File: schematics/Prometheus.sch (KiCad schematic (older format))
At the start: 15 parts, among them J1 ATX Power Conn, SW2 Power Switch, U1 wdc65c816, U2 DS1501YN, X1 8MHz, X2 32kHz

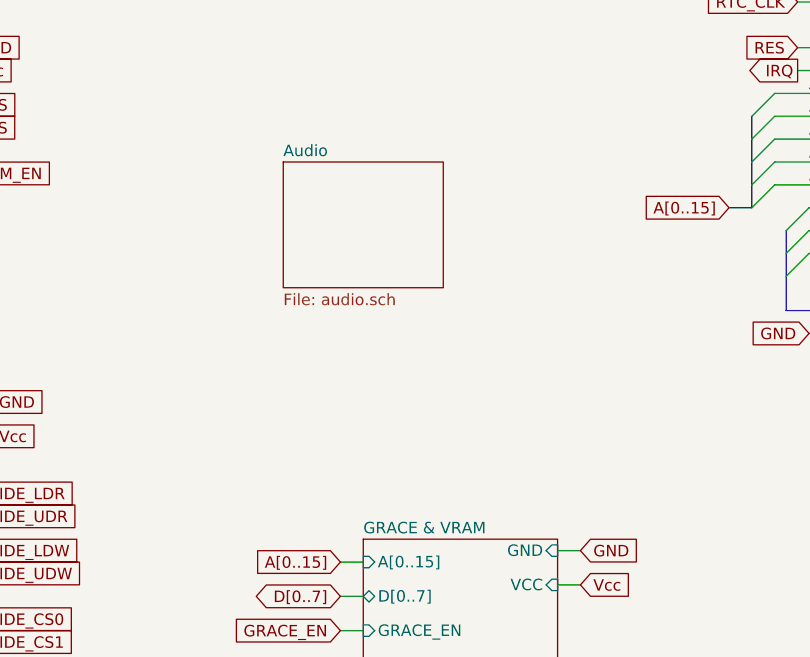
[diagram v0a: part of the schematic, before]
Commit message: finish up hierarchial pins (as they stand now)
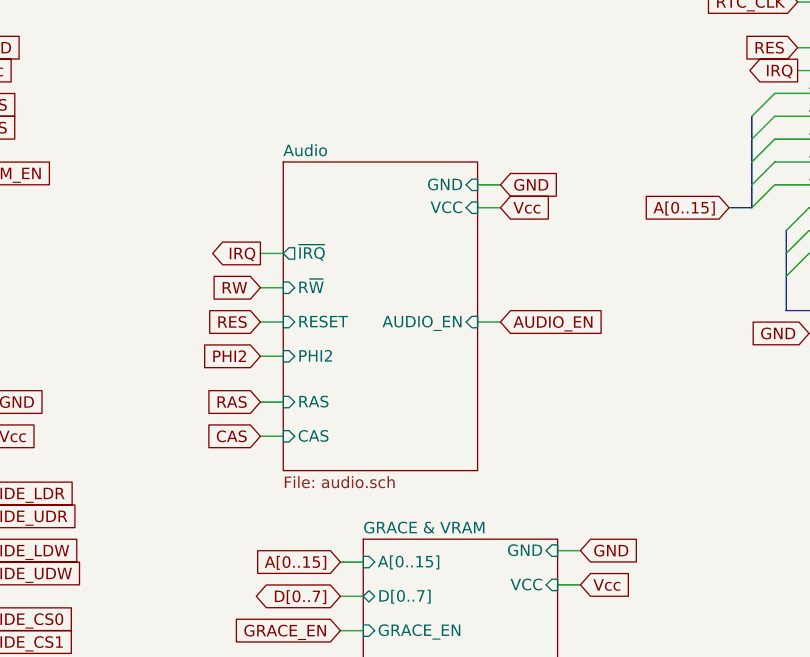
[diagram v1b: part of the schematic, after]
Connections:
- wire segments 197 -> 206
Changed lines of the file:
@@
 D7
 $Sheet
-S 3600 1850 700  550
+S 3600 1850 850  1350
 U 5F16299B
 F0 "Audio" 50
 F1 "audio.sch" 50
+F2 "AUDIO_EN" I R 4450 2550 50
+F3 "R~W" I L 3600 2400 50
+F4 "~IRQ" O L 3600 2250 50
+F5 "RESET" I L 3600 2550 50
+F6 "PHI2" I L 3600 2700 50
+F7 "RAS" I L 3600 2900 50
+F8 "CAS" I L 3600 3050 50
+F9 "VCC" I R 4450 2050 50
+F10 "GND" I R 4450 1950 50
 $EndSheet
 Text GLabel 10000 1650 2    50   Output ~ 0
@@
 Wire Wire Line
 	5750 5900 5850 5900
-Wire Bus Line
-	5800 2150 5800 2500
-Wire Bus Line
-	7050 2050 7050 2500
-Wire Bus Line
-	5650 1650 5650 2050
-Wire Bus Line
-	9950 2650 9950 3150
-Wire Bus Line
-	10100 1850 10100 2650
-Wire Bus Line
-	8500 1950 8500 3150
 Text GLabel 2250 5850 2    50   Output ~ 0
 VIA1_EN
@@
 Text GLabel 2250 6650 2    50   Output ~ 0
 IDE_EN
+Wire Wire Line
+	4450 1950 4550 1950
+Wire Wire Line
+	4450 2050 4550 2050
+Wire Wire Line
+	4450 2550 4550 2550
+Wire Wire Line
+	3600 2250 3500 2250
+Wire Wire Line
+	3600 2400 3500 2400
+Wire Wire Line
+	3600 2550 3500 2550
+Wire Wire Line
+	3600 2700 3500 2700
+Wire Wire Line
+	3600 2900 3500 2900
+Wire Wire Line
+	3600 3050 3500 3050
+Wire Bus Line
+	5800 2150 5800 2500
+Wire Bus Line
+	7050 2050 7050 2500
+Wire Bus Line
+	5650 1650 5650 2050
+Wire Bus Line
+	9950 2650 9950 3150
+Wire Bus Line
+	10100 1850 10100 2650
+Wire Bus Line
+	8500 1950 8500 3150
+Text GLabel 4550 1950 2    50   Input ~ 0
+GND
+Text GLabel 4550 2050 2    50   Input ~ 0
+Vcc
+Text GLabel 3500 2400 0    50   Input ~ 0
+RW
+Text GLabel 3500 2250 0    50   Output ~ 0
+IRQ
+Text GLabel 3500 2700 0    50   Input ~ 0
+PHI2
+Text GLabel 3500 2550 0    50   Input ~ 0
+RES
+Text GLabel 4550 2550 2    50   Input ~ 0
+AUDIO_EN
+Text GLabel 3500 3050 0    50   Input ~ 0
+CAS
+Text GLabel 3500 2900 0    50   Input ~ 0
+RAS
 $EndSCHEMATC
